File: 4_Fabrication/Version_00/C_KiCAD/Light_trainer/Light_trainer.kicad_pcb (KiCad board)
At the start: 2 copper layers, 70 parts, among them J1 USB_B_Micro, J2 Conn_01x02_Batterie, Q1 DMG3414U, Q2 S8050, Q3 S8050, SW1 SW_Push, SW2 SW_Push, SW3 SW_Push, SW4 SW_Push, SW5 SW_Push, SW6 SW_DIP_x04, SW7 SW_Push, U1 MCP73831-2-OT, U2 ESP32-WROOM-32, U3 LTC3525-5, U4 AP2112K-3.3, U5 CP2104

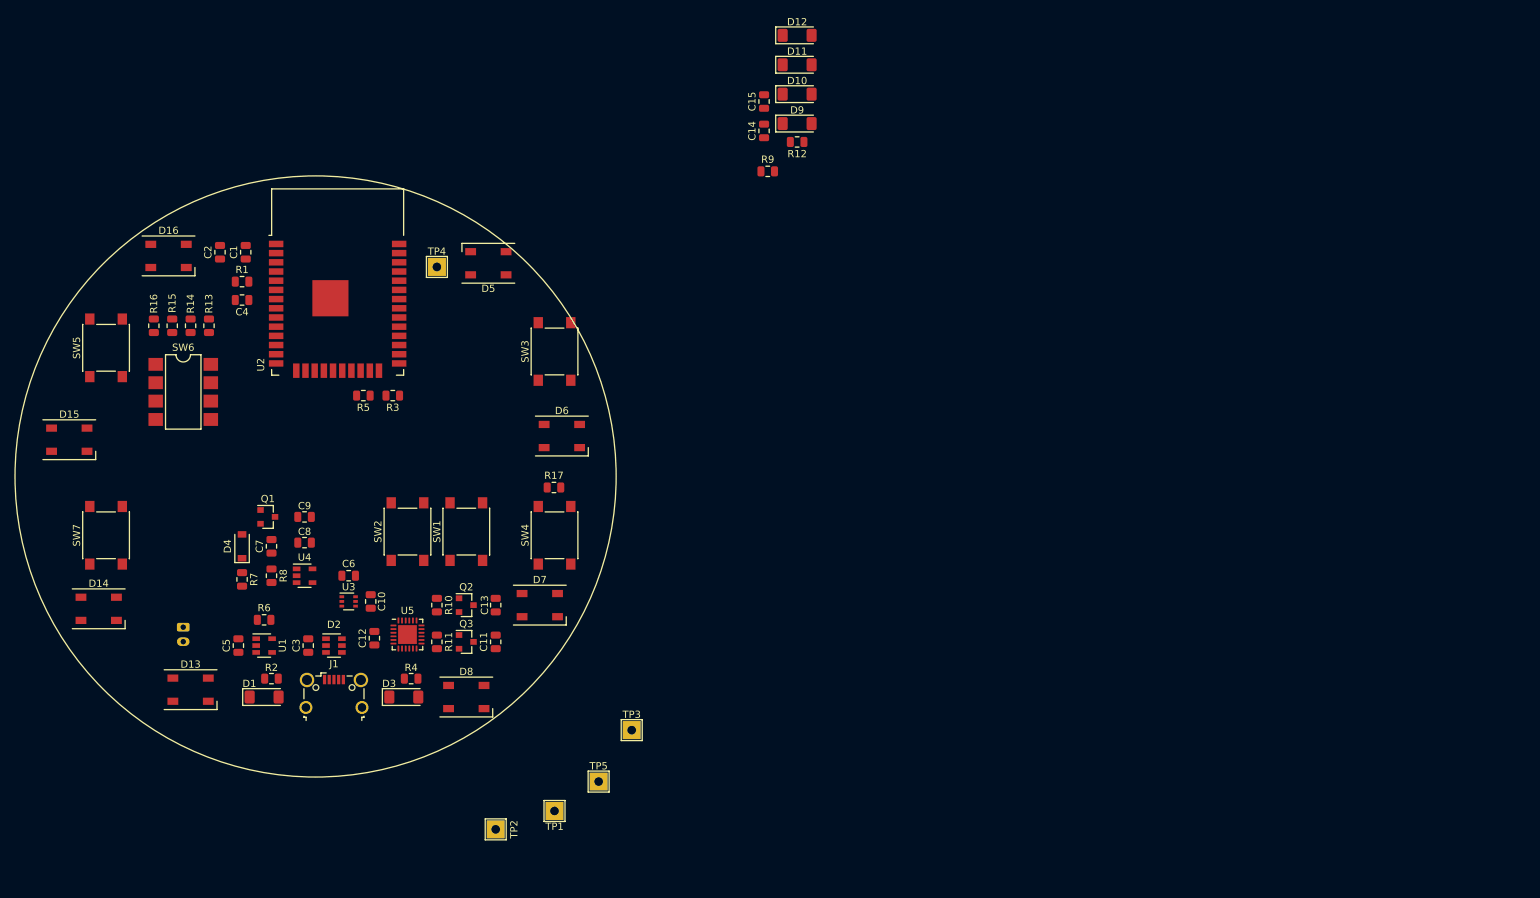
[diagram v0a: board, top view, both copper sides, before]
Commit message: modif kicad
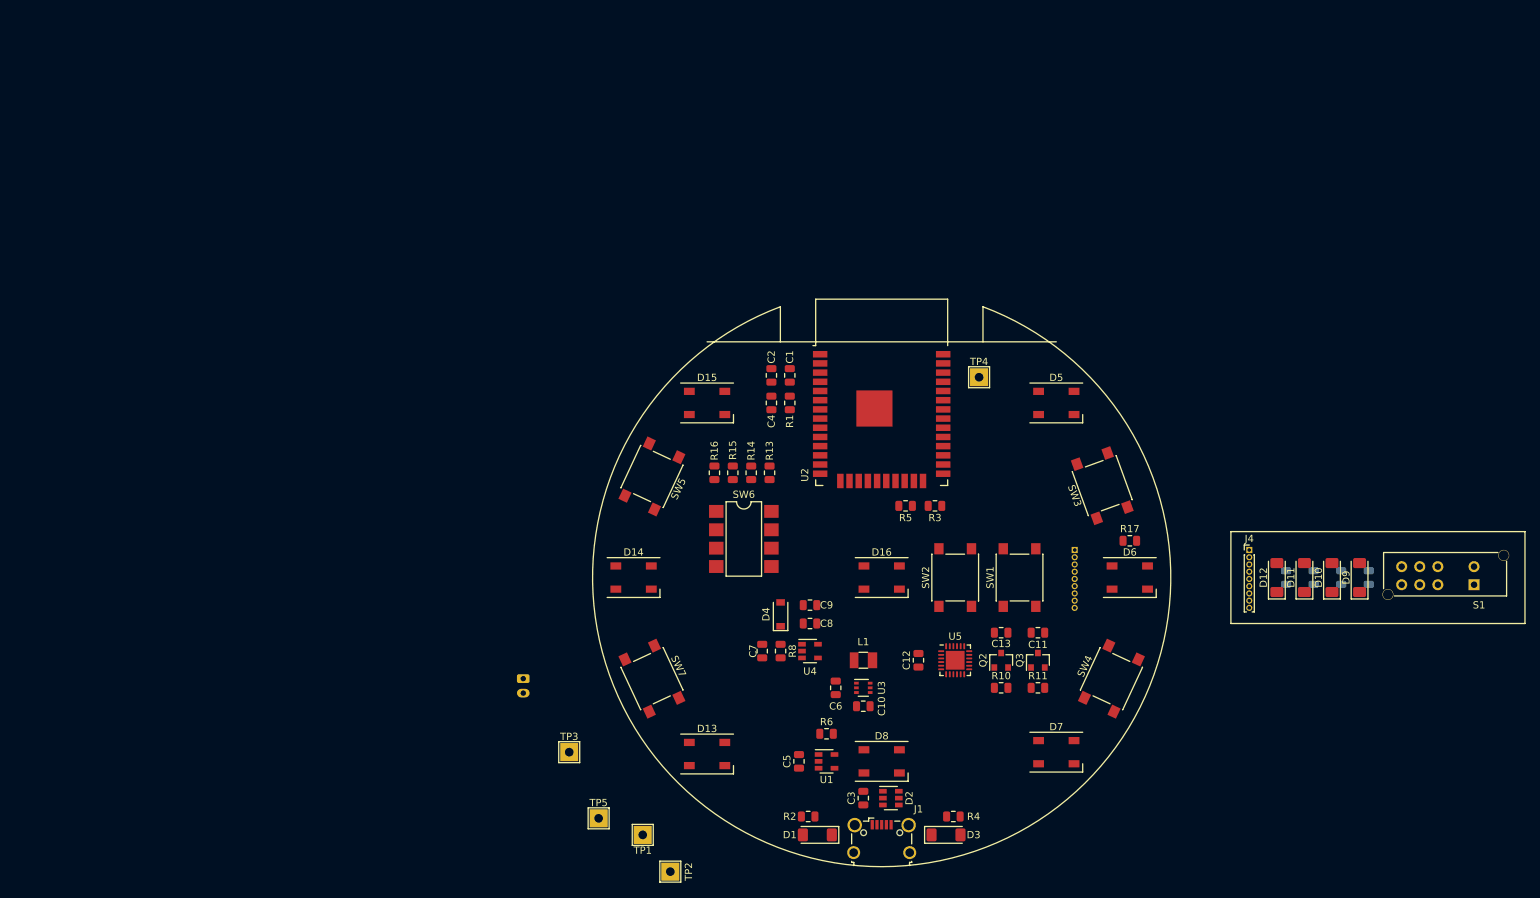
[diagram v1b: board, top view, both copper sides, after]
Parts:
- removed Q1: DMG3414U, Package_TO_SOT_SMD:SOT-23
- removed R7: 100k, Resistor_SMD:R_0805_2012Metric
- added J3: Conn_01x09_Female, Connector_PinHeader_1.00mm:PinHeader_1x09_P1.00mm_Vertical, B.Cu at (199.4, 96.5)
- added J4: Conn_01x09_Female, Connector_PinHeader_1.00mm:PinHeader_1x09_P1.00mm_Vertical, F.Cu at (223.5, 96.5)
- added L1: 10uH, Inductor_SMD:L_Wuerth_WE_PMI, F.Cu at (170.2, 111.8)
- added S1: SW_DP3T, Button_Switch_THT:SW_DP3T, F.Cu at (259.1, 102.9)
- C14, C15, R12, R9: moved to B.Cu
- C9: value 10uF -> 1uF
- moved D16 108.1 mm to (172.7, 100.3)
- moved C15 106.4 mm to (240.0, 100.3), turned to 270 degrees
- moved C14 100.8 mm to (236.2, 100.3)
- moved D12 100.0 mm to (227.3, 100.3), turned to 90 degrees
- moved D9 99.9 mm to (238.8, 100.3), turned to 90 degrees
- moved D11 99.7 mm to (231.1, 100.3), turned to 90 degrees
- moved D10 99.6 mm to (234.9, 100.3), turned to 90 degrees
- moved R12 93.4 mm to (232.4, 100.3), turned to 270 degrees
- moved R9 91.0 mm to (228.6, 100.3), turned to 270 degrees
- moved D15 88.3 mm to (148.6, 76.2)
- moved R11 83.3 mm to (194.3, 115.6), turned to 0 degrees
- moved D6 80.9 mm to (207.0, 100.3)
- moved D5 80.8 mm to (196.8, 76.2), turned to 0 degrees
- moved R14 80.1 mm to (154.7, 85.9)
- moved R13 80.1 mm to (157.2, 85.9)
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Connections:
- D4 pad 2: VBUS -> batt_on
- R9 pad 1: (no net) -> Net-(R9-Pad1)
- U2 pad 23: (no net) -> info_batt
- U3 pad 6: (no net) -> Net-(L1-Pad1)
